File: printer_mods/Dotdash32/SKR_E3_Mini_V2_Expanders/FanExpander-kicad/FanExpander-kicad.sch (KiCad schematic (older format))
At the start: 69 parts, among them J0 JST-XH2, J1 JST-XH2, J10 JST-XH2, J12 HI_PWR2, J2 JST-XH2, J3 JST-XH2, J4 JST-XH2, J5 JST-XH2, J6 JST-XH2, J7 JST-XH2, J8 EXPx_IN, J9 5V_In, Q1 IRLML6344, Q2 IRLML6344, Q3 IRLML6344, Q4 IRLML6344, Q5 IRLML6344, Q6 IRLML6344, Q7 IRLML6344

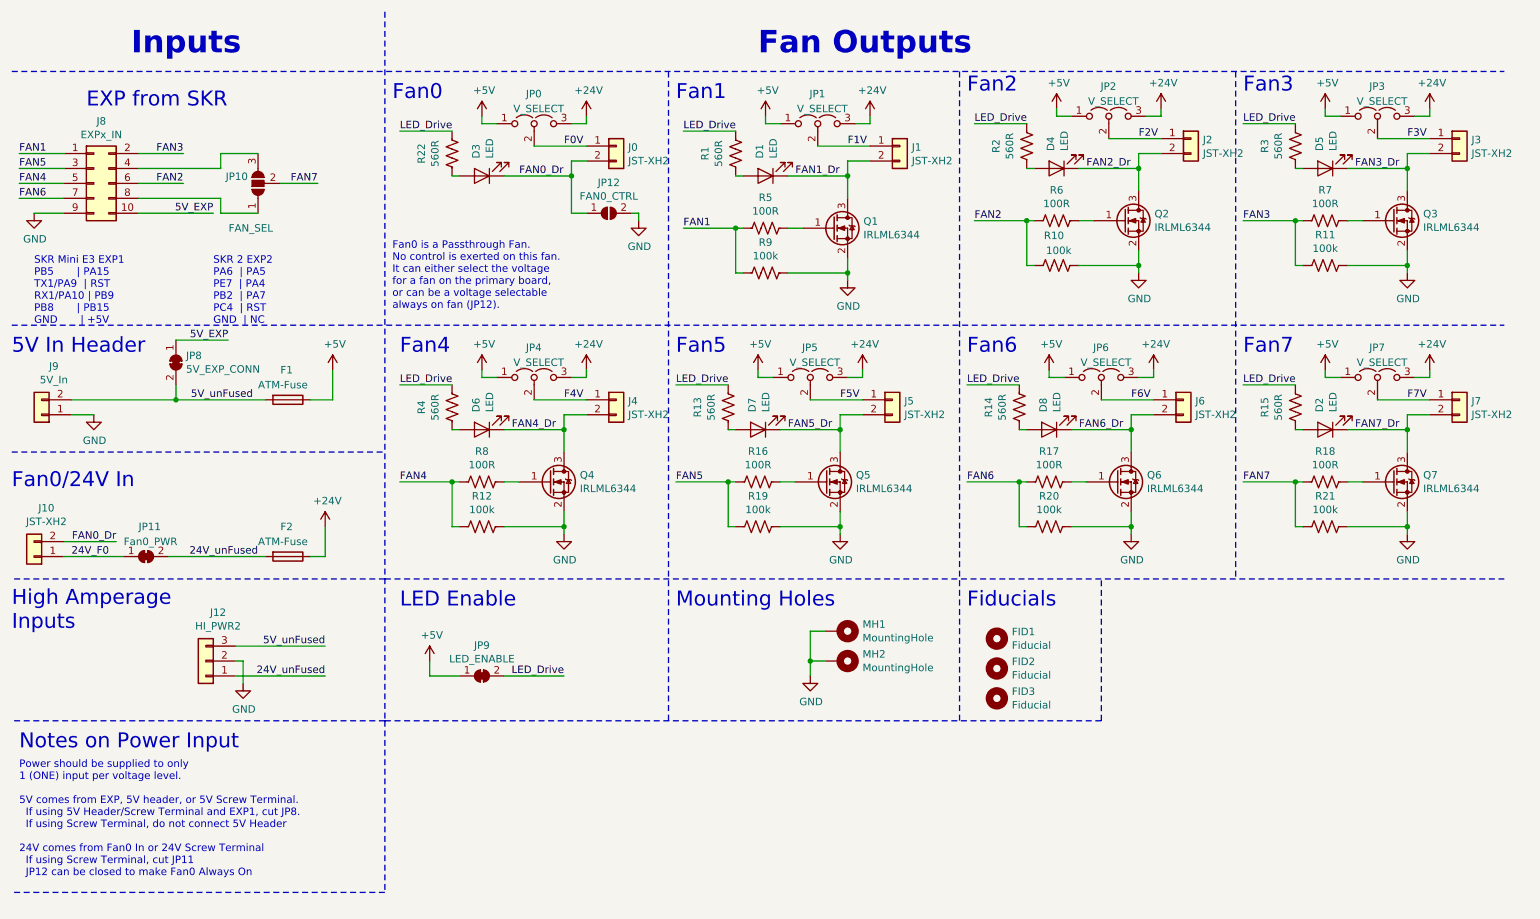
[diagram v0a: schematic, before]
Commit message: feat: prep big expander for release
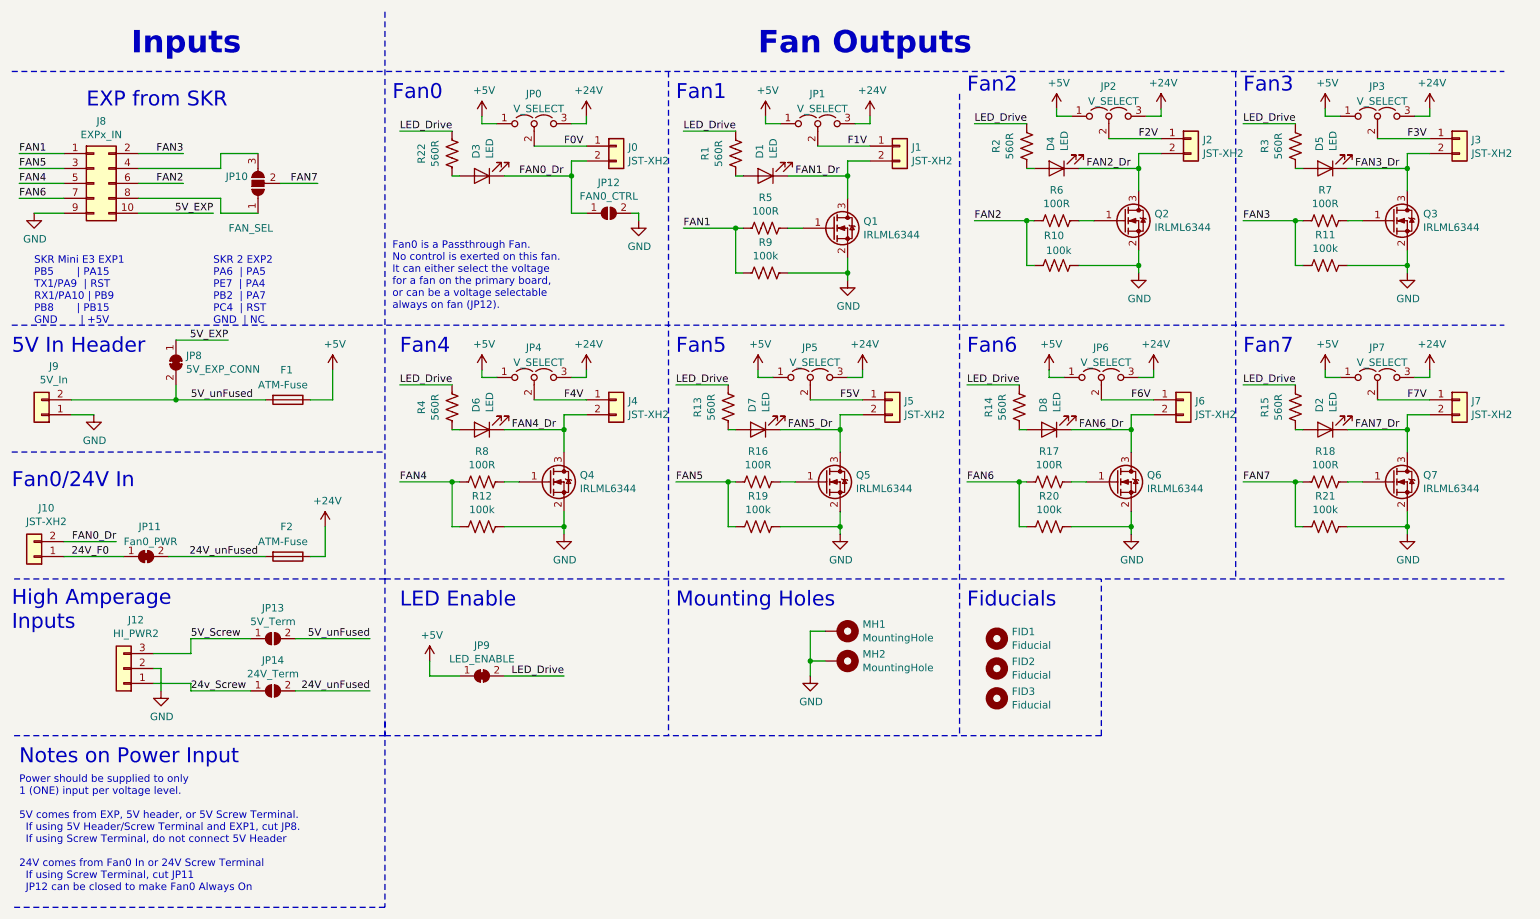
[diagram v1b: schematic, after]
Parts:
- added JP13: 5V_Term, Jumper:SolderJumper-2_P1.3mm_Open_RoundedPad1.0x1.5mm, symbol Jumper:SolderJumper_2_Open
- added JP14: 24V_Term, Jumper:SolderJumper-2_P1.3mm_Open_RoundedPad1.0x1.5mm, symbol Jumper:SolderJumper_2_Open
- JP11, JP8, JP9: footprint Jumper:SolderJumper-2_P1.3mm_Bridged_RoundedPad1.0x1.5mm -> Jumper:SolderJumper-2_P1.3mm_Pasted_RoundedPad1.0x1.5mm
- JP12: footprint Jumper:SolderJumper-2_P1.3mm_Bridged2Bar_RoundedPad1.0x1.5mm -> Jumper:SolderJumper-2_P1.3mm_Open_RoundedPad1.0x1.5mm
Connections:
- net 24V_unFused: now also JP14.2 (B); no longer J12.1 (Pin_1)
- net 5V_unFused: now also JP13.2 (B); no longer J12.3 (Pin_3)
- new net 24v_Screw: J12.1 (Pin_1), JP14.1 (A)
- new net 5V_Screw: J12.3 (Pin_3), JP13.1 (A)
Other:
- moved on the sheet: J12
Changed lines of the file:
@@
 Sheet 1 1
 Title "SKR Fan Expander"
-Date "2022-01-14"
-Rev "V0.1.5"
+Date "2022-01-16"
+Rev "V1.0.1"
 Comp "Voron Design"
 Comment1 "Drawn by Dotdash32 (JDeW)"
@@
 F 0 "JP9" H 3650 5155 50  0000 C CNN
 F 1 "LED_ENABLE" H 3650 5064 50  0000 C CNN
-F 2 "Jumper:SolderJumper-2_P1.3mm_Bridged_RoundedPad1.0x1.5mm" H 3650 4950 50  0001 C CNN
+F 2 "Jumper:SolderJumper-2_P1.3mm_Pasted_RoundedPad1.0x1.5mm" H 3650 4950 50  0001 C CNN
 F 3 "~" H 3650 4950 50  0001 C CNN
 	1    3650 4950
@@
 Connection ~ 5850 4850
 Wire Notes Line
-	4900 900  4900 5250
+	4900 900  4900 5350
 Wire Notes Line
-	6850 900  6850 5250
+	6850 1050 6850 5350
 Text Notes 4950 4500 0    100  ~ 0
 Mounting Holes
@@
 	3000 4300 500  4300
 Wire Notes Line width 12 style solid
-	3000 5250 500  5250
+	3000 5350 500  5350
 Wire Notes Line width 12 style solid
-	3000 500  3000 5250
+	3000 500  3000 5350
 Text Label 1950 2700 2    50   ~ 0
 5V_EXP
@@
 F 0 "JP8" V 1554 2918 50  0000 L CNN
 F 1 "5V_EXP_CONN" V 1645 2918 50  0000 L CNN
-F 2 "Jumper:SolderJumper-2_P1.3mm_Bridged_RoundedPad1.0x1.5mm" H 1600 2850 50  0001 C CNN
+F 2 "Jumper:SolderJumper-2_P1.3mm_Pasted_RoundedPad1.0x1.5mm" H 1600 2850 50  0001 C CNN
 F 3 "~" H 1600 2850 50  0001 C CNN
 	1    1600 2850
@@
 F 0 "JP12" H 4500 2055 50  0000 C CNN
 F 1 "FAN0_CTRL" H 4500 1964 50  0000 C CNN
-F 2 "Jumper:SolderJumper-2_P1.3mm_Bridged2Bar_RoundedPad1.0x1.5mm" H 4500 1850 50  0001 C CNN
+F 2 "Jumper:SolderJumper-2_P1.3mm_Open_RoundedPad1.0x1.5mm" H 4500 1850 50  0001 C CNN
 F 3 "~" H 4500 1850 50  0001 C CNN
 	1    4500 1850
@@
 L Connector_Generic:Conn_01x03 J12
 U 1 1 61F3F4E8
-P 1800 4850
-F 0 "J12" H 1718 4525 50  0000 C CNN
-F 1 "HI_PWR2" H 1718 4616 50  0000 C CNN
-F 2 "TerminalBlock_Pheonix:TerminalBlock_Phoenix_MKDS-1,5-3-5.08_1x03_P5.08mm_Horizontal" H 1800 4850 50  0001 C CNN
-F 3 "~" H 1800 4850 50  0001 C CNN
-	1    1800 4850
+P 1250 4900
+F 0 "J12" H 1168 4575 50  0000 C CNN
+F 1 "HI_PWR2" H 1168 4666 50  0000 C CNN
+F 2 "TerminalBlock_Pheonix:TerminalBlock_Phoenix_MKDS-1,5-3-5.08_1x03_P5.08mm_Horizontal" H 1250 4900 50  0001 C CNN
+F 3 "~" H 1250 4900 50  0001 C CNN
+	1    1250 4900
 	-1   0    0    1
 $EndComp
@@
 L power:GND #PWR0108
 U 1 1 61FA64D9
-P 2050 5000
-F 0 "#PWR0108" H 2050 4750 50  0001 C CNN
-F 1 "GND" H 2055 4827 50  0000 C CNN
-F 2 "" H 2050 5000 50  0001 C CNN
-F 3 "" H 2050 5000 50  0001 C CNN
-	1    2050 5000
-	1    0    0    -1
-$EndComp
-Wire Wire Line
-	2000 4850 2050 4850
-Wire Wire Line
-	2000 4950 2600 4950
-Wire Wire Line
-	2000 4750 2600 4750
-Text Label 2600 4750 2    50   ~ 0
+P 1500 5050
+F 0 "#PWR0108" H 1500 4800 50  0001 C CNN
+F 1 "GND" H 1505 4877 50  0000 C CNN
+F 2 "" H 1500 5050 50  0001 C CNN
+F 3 "" H 1500 5050 50  0001 C CNN
+	1    1500 5050
+	1    0    0    -1
+$EndComp
+Wire Wire Line
+	1450 4900 1500 4900
+Text Label 2900 4700 2    50   ~ 0
 5V_unFused
-Text Label 2600 4950 2    50   ~ 0
+Text Label 2900 5050 2    50   ~ 0
 24V_unFused
 Wire Wire Line
-	2050 5000 2050 4850
-Text Notes 550  6300 0    50   ~ 0
+	1500 5050 1500 4900
+Text Notes 550  6400 0    50   ~ 0
 Power should be supplied to only \n1 (ONE) input per voltage level.\n\n5V comes from EXP, 5V header, or 5V Screw Terminal.\n  If using 5V Header/Screw Terminal and EXP1, cut JP8.\n  If using Screw Terminal, do not connect 5V Header\n\n24V comes from Fan0 In or 24V Screw Terminal\n  If using Screw Terminal, cut JP11\n  JP12 can be closed to make Fan0 Always On
 $Comp
@@
 F 0 "JP11" H 1350 4350 50  0000 L CNN
 F 1 "Fan0_PWR" H 1250 4250 50  0000 L CNN
-F 2 "Jumper:SolderJumper-2_P1.3mm_Bridged_RoundedPad1.0x1.5mm" H 1400 4150 50  0001 C CNN
+F 2 "Jumper:SolderJumper-2_P1.3mm_Pasted_RoundedPad1.0x1.5mm" H 1400 4150 50  0001 C CNN
 F 3 "~" H 1400 4150 50  0001 C CNN
 	1    1400 4150
@@
 Text Label 900  4150 0    50   ~ 0
 24V_F0
-Text Notes 550  5450 0    100  ~ 0
+Text Notes 550  5550 0    100  ~ 0
 Notes on Power Input
 Wire Notes Line
-	3000 5250 3000 6400
+	3000 5250 3000 6500
 Wire Notes Line
-	3000 6400 500  6400
+	3000 6500 500  6500
 $Comp
 L Mechanical:MountingHole FID1
@@
 Fiducials
 Wire Notes Line
-	7800 5250 7800 4300
+	7800 5350 7800 4300
 Wire Notes Line
-	3000 5250 7800 5250
+	3000 5350 7800 5350
+$Comp
+L Jumper:SolderJumper_2_Open JP13
+U 1 1 61EEFF27
+P 2250 4700
+F 0 "JP13" H 2250 4905 50  0000 C CNN
+F 1 "5V_Term" H 2250 4814 50  0000 C CNN
+F 2 "Jumper:SolderJumper-2_P1.3mm_Open_RoundedPad1.0x1.5mm" H 2250 4700 50  0001 C CNN
+F 3 "~" H 2250 4700 50  0001 C CNN
+	1    2250 4700
+	1    0    0    -1
+$EndComp
+$Comp
+L Jumper:SolderJumper_2_Open JP14
+U 1 1 61EF10E8
+P 2250 5050
+F 0 "JP14" H 2250 5255 50  0000 C CNN
+F 1 "24V_Term" H 2250 5164 50  0000 C CNN
+F 2 "Jumper:SolderJumper-2_P1.3mm_Open_RoundedPad1.0x1.5mm" H 2250 5050 50  0001 C CNN
+F 3 "~" H 2250 5050 50  0001 C CNN
+	1    2250 5050
+	1    0    0    -1
+$EndComp
+Wire Wire Line
+	2900 4700 2400 4700
+Wire Wire Line
+	1450 5000 1700 5000
+Wire Wire Line
+	1700 5000 1700 5050
+Wire Wire Line
+	1700 5050 2100 5050
+Wire Wire Line
+	1450 4800 1700 4800
+Wire Wire Line
+	1700 4800 1700 4700
+Wire Wire Line
+	1700 4700 2100 4700
+Wire Wire Line
+	2400 5050 2900 5050
+Text Label 1700 4700 0    50   ~ 0
+5V_Screw
+Text Label 1700 5050 0    50   ~ 0
+24v_Screw
 $EndSCHEMATC
